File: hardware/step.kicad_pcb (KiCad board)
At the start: 4 copper layers, 150 x 35 mm, 127 parts, among them J101 WAGO 2065-100, J102 WAGO 2065-100, J103 Cortex_Debug, J1901 2x05_Horizontal, J2001 2x05_Horizontal, J201 WAGO 2065-100, J202 WAGO 2065-100, J203 WAGO 2065-100, J204 WAGO 2065-100, J301 WAGO 2065-100, J302 WAGO 2065-100, J303 WAGO 2065-100, J304 WAGO 2065-100, J401 WAGO 2065-100, J402 WAGO 2065-100, J403 WAGO 2065-100, J404 WAGO 2065-100, J501 WAGO 2065-100, J502 WAGO 2065-100, J503 WAGO 2065-100, J504 WAGO 2065-100, SW101 SKSG, SW102 SKSG, U101 ATSAMD51J, U102 TPS78433QWDRBRQ1, U1901 THVD2442, U2001 THVD2442, U201 TMC2130-LA, U301 TMC2130-LA, U401 TMC2130-LA, U501 TMC2130-LA, Y101 32k768

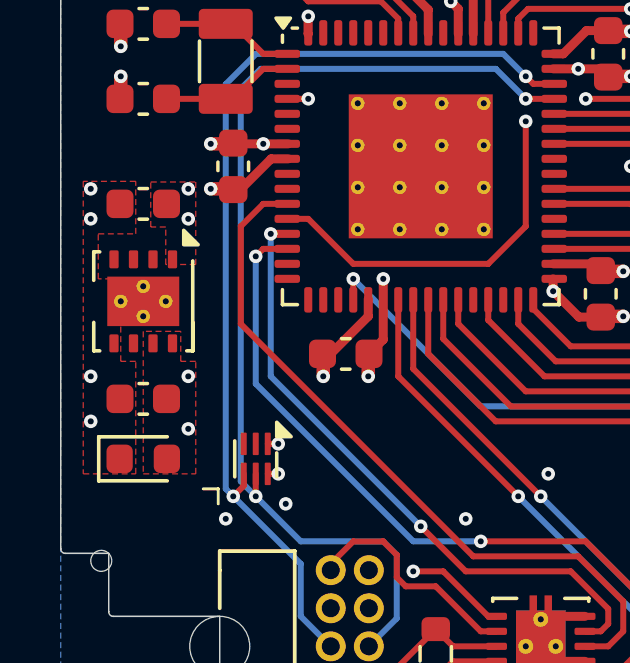
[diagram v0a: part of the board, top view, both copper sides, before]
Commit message: Update parts
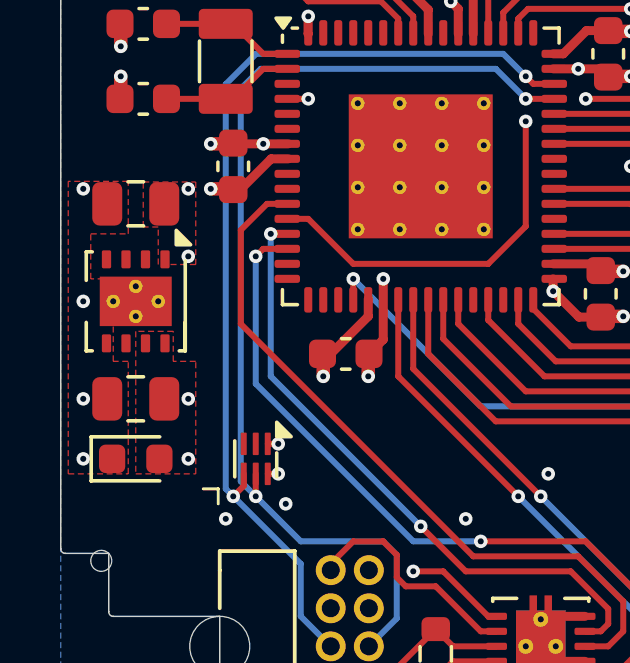
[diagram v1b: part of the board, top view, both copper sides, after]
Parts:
- C110, C111: footprint V2_Capacitor_SMD:C_0603 -> V2_Capacitor_SMD:C_0805
- C206, C306, C406, C506: value 0u470 -> 0u47
- moved C110 0.25 mm to (79.5, 101.2)
- moved C111 0.25 mm to (79.5, 94.8)
- moved TVS102 0.25 mm to (79.5, 103.2)
- moved U102 0.25 mm to (79.5, 98.0)
